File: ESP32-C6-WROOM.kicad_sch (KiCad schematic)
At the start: 42 parts, among them J1 Conn_01x04, J2 USB_C_Receptacle_USB2.0_16P, J3 Pin 2x5, J4 Pin 2x3, SW1 SW_SPST, SW2 SW_SPST, SW3 SW_SPST, U1 LM1117MP-3.3, U2 HDC3022QDEJRQ1, U3 USBLC6-2SC6, U4 ESP32-C6-WROOM-1

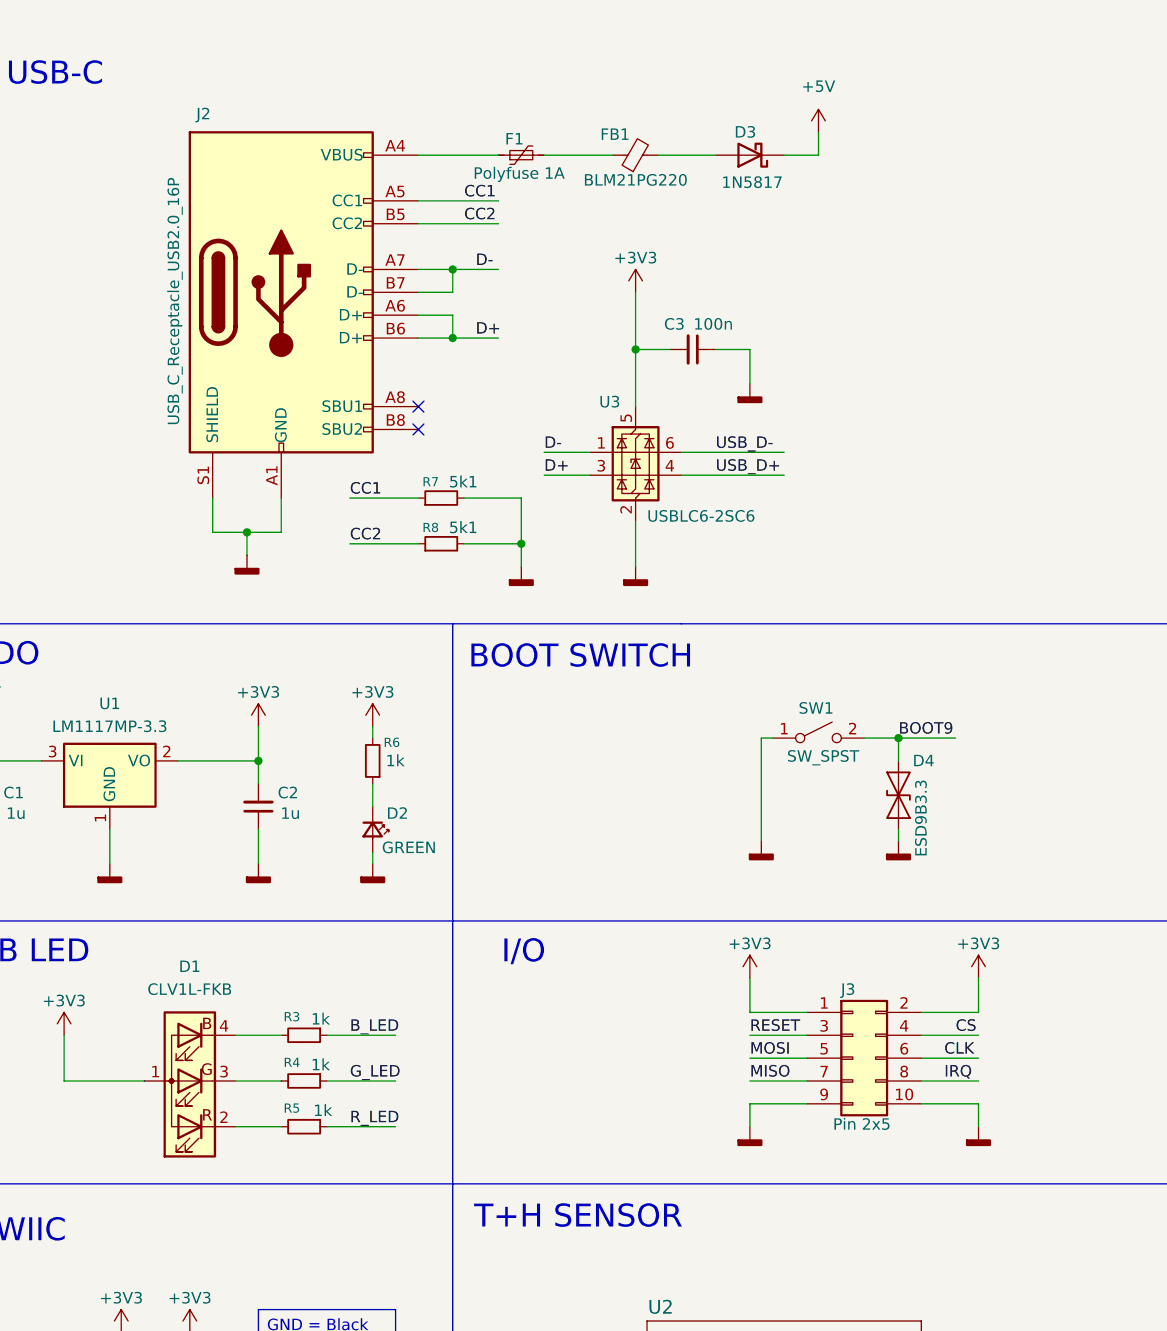
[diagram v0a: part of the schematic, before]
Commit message: auto backup
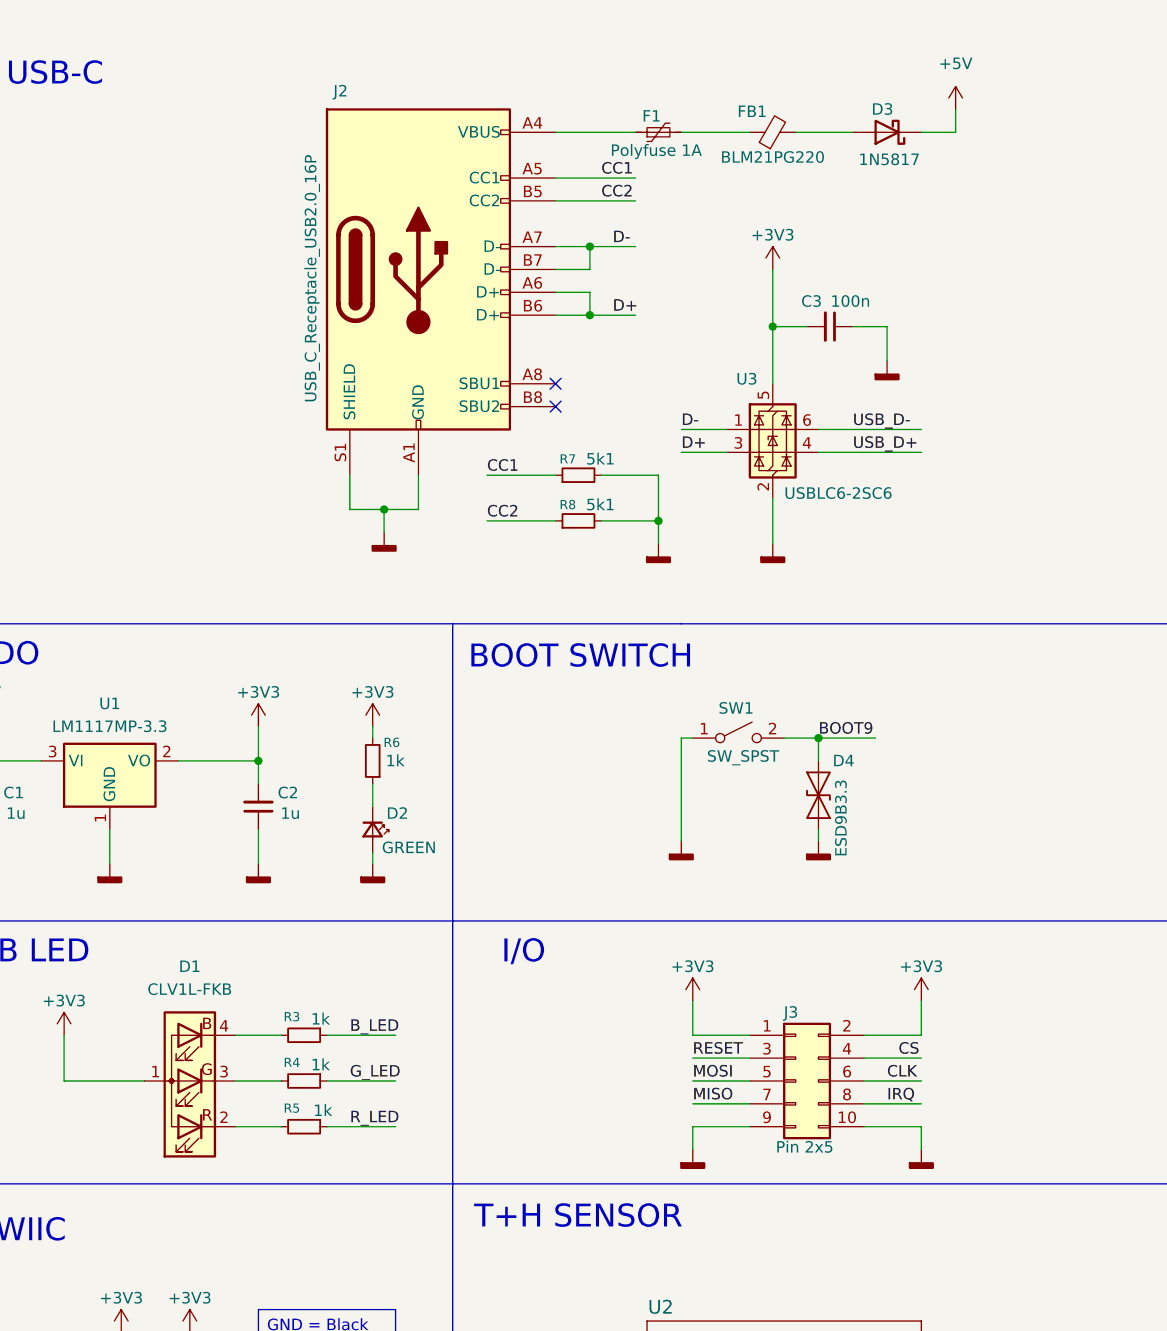
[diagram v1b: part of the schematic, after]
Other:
- moved on the sheet: C3, D3, D4, F1, FB1, J2, J3, R7, R8, SW1, U3
